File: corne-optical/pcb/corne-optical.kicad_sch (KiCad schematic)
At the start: 62 parts, among them J1 MJ-4PP-9, J2 Conn_01x04, J3 Conn_01x03, J4 Conn_01x01, J4 Conn_01x02, J5 Conn_01x01, J5 Conn_01x02, Q1 Q_NMOS_GSD, Q2 Q_NMOS_GSD, Q3 Q_NMOS_GSD, Q4 Q_NMOS_GSD, Q5 Q_NMOS_GSD, Q6 Q_NMOS_GSD, SW1 Keychron_LP_Optical, SW10 Keychron_LP_Optical, SW11 Keychron_LP_Optical, SW12 Keychron_LP_Optical, SW13 Keychron_LP_Optical, SW14 Keychron_LP_Optical, SW15 Keychron_LP_Optical, SW16 Keychron_LP_Optical, SW17 Keychron_LP_Optical, SW18 Keychron_LP_Optical, SW19 Keychron_LP_Optical, SW2 Keychron_LP_Optical, SW20 Keychron_LP_Optical, SW21 Keychron_LP_Optical, SW3 Keychron_LP_Optical, SW4 Keychron_LP_Optical, SW5 Keychron_LP_Optical, SW6 Keychron_LP_Optical, SW7 Keychron_LP_Optical, SW8 Keychron_LP_Optical, SW9 Keychron_LP_Optical, U1 ProMicro

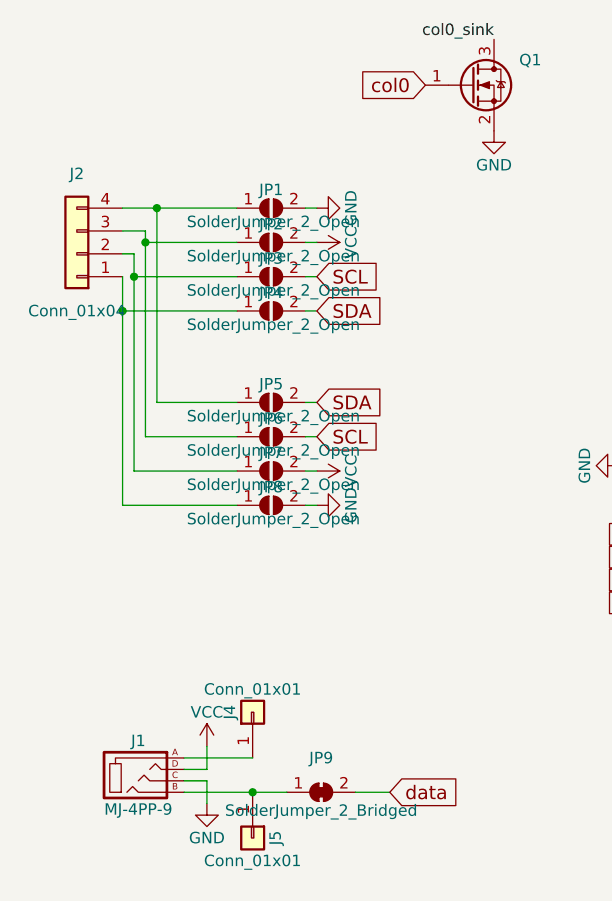
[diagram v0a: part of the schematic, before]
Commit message: Missed a few
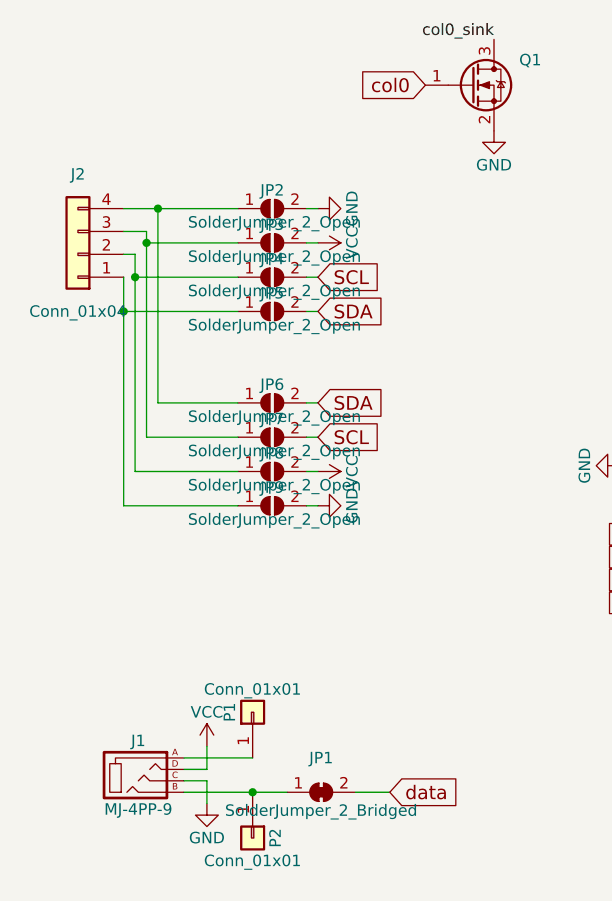
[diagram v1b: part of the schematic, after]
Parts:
- renumbered JP9 to JP1, JP1 to JP9, J4 to P1, J5 to P2
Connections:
- net GND: now also JP2.2 (B); no longer JP8.2 (B)
- net SCL: now also JP4.2 (B), JP7.2 (B); no longer JP3.2 (B), JP6.2 (B)
- net SDA: now also JP6.2 (B); no longer JP4.2 (B)
- net VCC: now also JP3.2 (B), JP8.2 (B); no longer JP2.2 (B), JP7.2 (B)
- net at JP4.1 (A), JP8.1 (A): now also J2.2 (Pin_2); no longer J2.1 (Pin_1)
- net at JP3.1 (A), JP7.1 (A): now also J2.3 (Pin_3); no longer J2.2 (Pin_2)
- net at JP2.1 (A), JP6.1 (A): now also J2.4 (Pin_4); no longer J2.3 (Pin_3)
- net at JP5.1 (A), JP9.1 (A): now also J2.1 (Pin_1); no longer J2.4 (Pin_4)
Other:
- moved on the sheet: JP2, JP3, JP4, JP5, JP6, JP7, JP8, JP9

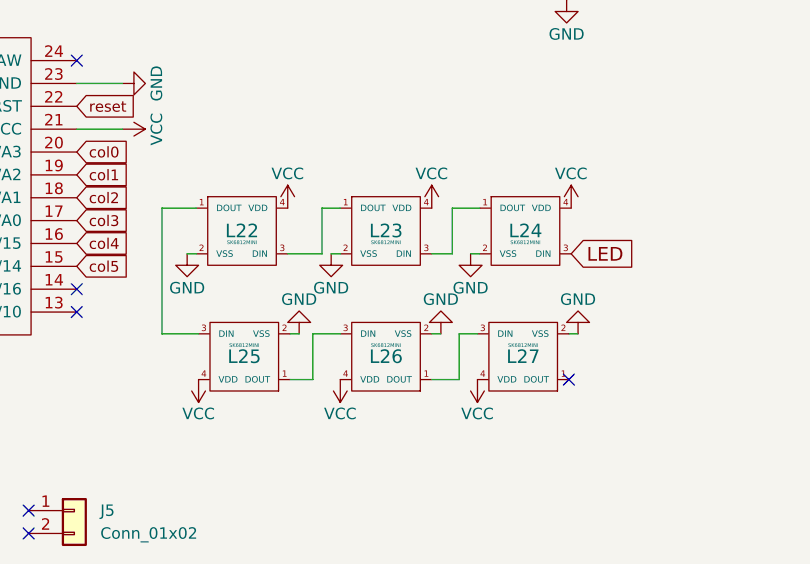
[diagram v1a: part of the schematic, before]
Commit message: Trying to workout phantom copper
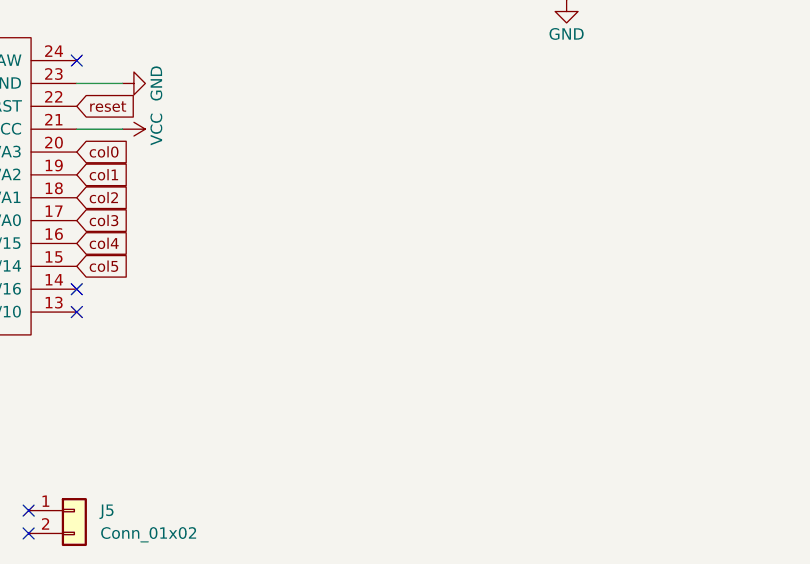
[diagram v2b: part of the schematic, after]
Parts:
- removed L22, L23, L24, L25, L26, L27: SK6812MINI, kbd:SK6812MINI_underglow_rev, symbol kbd:SK6812MINI
- SW1, SW10, SW11, SW12, SW13, SW14, SW15, SW16, SW17, SW18, SW19, SW2, SW20, SW3, SW4, SW5, SW6, SW7, SW8, SW9: footprint kbd:Choc_Hotswap -> optical:Keychron_LP_Optical
- SW21: footprint kbd:Choc_Hotswap_1.5u -> optical:Keychron_LP_Optical_1.5u
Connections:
- no-connect marks 10 -> 9
